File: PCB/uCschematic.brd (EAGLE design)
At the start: 90 x 80 mm, 63 parts, among them IC1 PIC24FJXXGA002/SO, IC10 ULN2003D1013TR, IC11 ULN2003D1013TR, IC12 ULN2003D1013TR, IC13 FT230XS-U, IC2 317EMP, IC3 MC74HC175ADG, IC4 MC74HC175ADG, IC5 MC74HC175ADG, IC6 MC74HC175ADG, IC7 MC74HC175ADG, IC8 MC74HC175ADG, IC9 ULN2003D1013TR, J1 UJ2-BH-1-TH, J8 68000-105HTLF, J9 68000-105HTLF, U1 74HC237D-Q100J

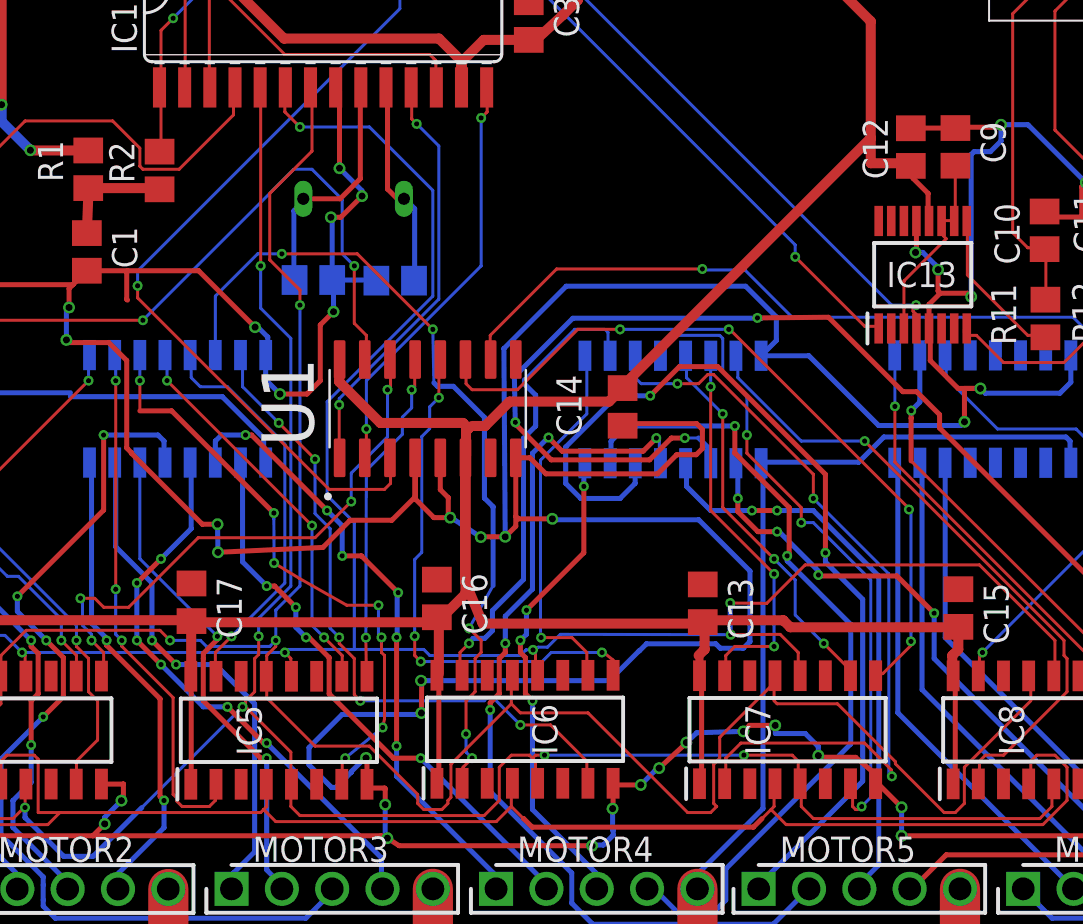
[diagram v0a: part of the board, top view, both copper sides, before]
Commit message: Ispravke u rutiranju
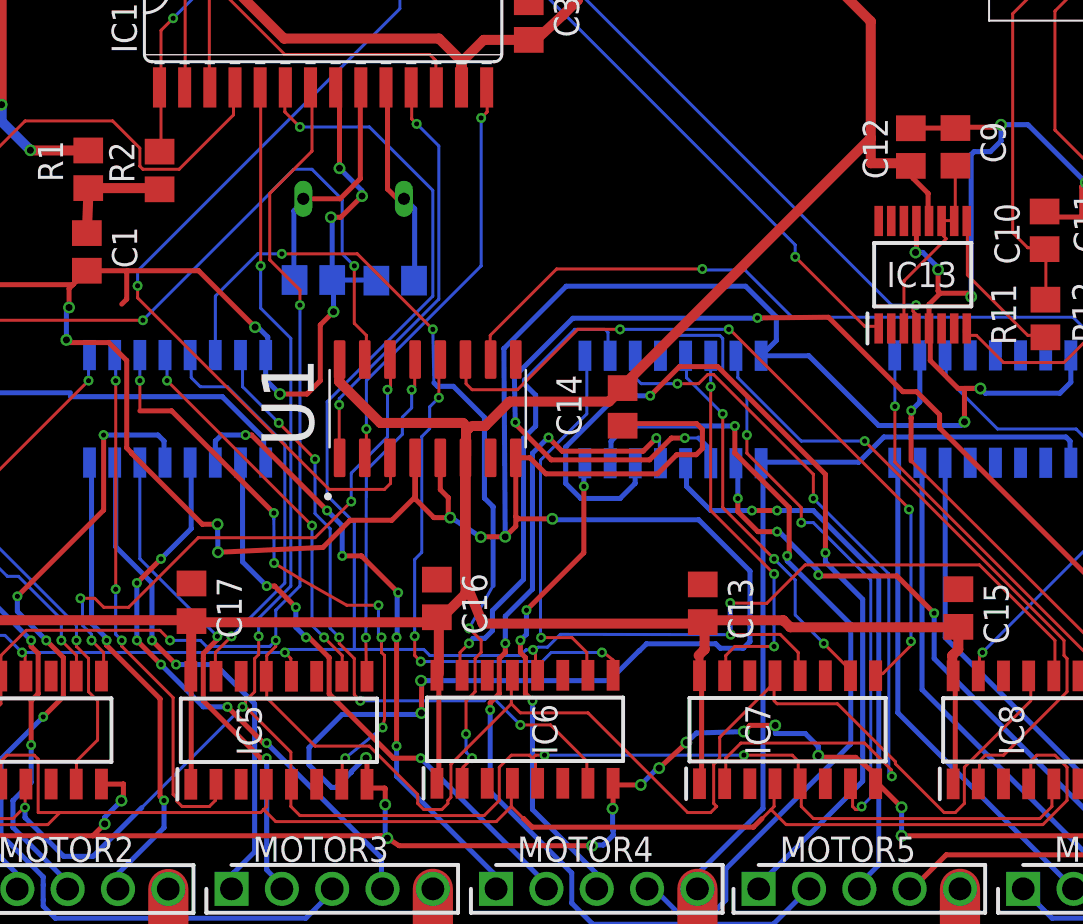
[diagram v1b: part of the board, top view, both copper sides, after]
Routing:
- net GND: track 500.6 -> 501.1 mm
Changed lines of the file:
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@@
 <?xml version="1.0" encoding="utf-8"?>
 <!DOCTYPE eagle SYSTEM "eagle.dtd">
-<eagle version="6.6.0">
+<eagle version="9.6.2">
 <drawing>
 <settings>
 <setting alwaysvectorfont="no"/>
+<setting keepoldvectorfont="yes"/>
 <setting verticaltext="up"/>
 </settings>
@@
 <param name="dpMaxLengthDifference" value="10mm"/>
 <param name="dpGapFactor" value="2.5"/>
-<param name="checkGrid" value="0"/>
 <param name="checkAngle" value="0"/>
 <param name="checkFont" value="1"/>
 <param name="checkRestrict" value="1"/>
+<param name="checkStop" value="0"/>
+<param name="checkValues" value="0"/>
+<param name="checkNames" value="1"/>
+<param name="checkWireStubs" value="1"/>
+<param name="checkPolygonWidth" value="0"/>
 <param name="useDiameter" value="13"/>
 <param name="maxErrors" value="50"/>
@@
 <pass name="Default">
 <param name="RoutingGrid" value="0.25mm"/>
+<param name="AutoGrid" value="1"/>
+<param name="Efforts" value="0"/>
+<param name="TopRouterVariant" value="1"/>
 <param name="tpViaShape" value="round"/>
 <param name="PrefDir.1" value="|"/>
@@
 <via x="20.20364375" y="9.065396875" extent="1-16" drill="0.35"/>
 <via x="27.5551375" y="9.661984375" extent="1-16" drill="0.35"/>
-<wire x1="28.39883125" y1="10.77141875" x2="28.39883125" y2="10.83833125" width="0.254" layer="16"/>
+<wire x1="28.39883125" y1="10.760046875" x2="28.39883125" y2="10.83833125" width="0.254" layer="16"/>
 <via x="28.39883125" y="10.83833125" extent="1-16" drill="0.35"/>
 <wire x1="28.39883125" y1="10.83833125" x2="28.49918125" y2="10.93868125" width="0.254" layer="1"/>
@@
 <wire x1="61.398775" y1="14.224465625" x2="61.3913375" y2="14.63620625" width="0.254" layer="16"/>
 <via x="61.3913375" y="14.63620625" extent="1-16" drill="0.35"/>
-<wire x1="59.676584375" y1="14.301878125" x2="59.7856" y2="14.33315" width="0.254" layer="1"/>
-<via x="59.7856" y="14.33315" extent="1-16" drill="0.35"/>
-<wire x1="59.7856" y1="14.33315" x2="57.432025" y2="14.263171875" width="0.254" layer="16"/>
-<wire x1="57.432025" y1="14.263171875" x2="56.906190625" y2="13.768446875" width="0.254" layer="16"/>
+<wire x1="59.693640625" y1="14.29050625" x2="59.80265625" y2="14.321778125" width="0.254" layer="1"/>
+<via x="59.80265625" y="14.321778125" extent="1-16" drill="0.35"/>
+<wire x1="59.80265625" y1="14.321778125" x2="57.4189875" y2="14.25090625" width="0.254" layer="16"/>
+<wire x1="57.4189875" y1="14.25090625" x2="56.906190625" y2="13.768446875" width="0.254" layer="16"/>
 <via x="56.906190625" y="13.768446875" extent="1-16" drill="0.35"/>
 <wire x1="56.906190625" y1="13.768446875" x2="56.75484375" y2="13.60516875" width="0.254" layer="1"/>
@@
 <wire x1="7.42666875" y1="57.50661875" x2="7.075165625" y2="57.858121875" width="0.254" layer="16"/>
 <wire x1="14.985165625" y1="47.508121875" x2="14.985165625" y2="49.41515" width="0.254" layer="16"/>
-<wire x1="61.3913375" y1="14.63620625" x2="60.08865625" y2="14.63620625" width="0.254" layer="1"/>
-<wire x1="60.08865625" y1="14.63620625" x2="59.7856" y2="14.33315" width="0.254" layer="1"/>
+<wire x1="61.3913375" y1="14.63620625" x2="60.117084375" y2="14.63620625" width="0.254" layer="1"/>
+<wire x1="60.117084375" y1="14.63620625" x2="59.80265625" y2="14.321778125" width="0.254" layer="1"/>
 <wire x1="15.005165625" y1="44.008121875" x2="15.005165625" y2="41.4866625" width="0.254" layer="16"/>
 <wire x1="15.005165625" y1="41.4866625" x2="15.055459375" y2="41.43636875" width="0.254" layer="16"/>
@@
 <wire x1="78.385225" y1="42.92861875" x2="78.385225" y2="46.080515625" width="0.254" layer="1"/>
 <wire x1="78.385225" y1="46.080515625" x2="82.582053125" y2="50.27734375" width="0.254" layer="1"/>
-<wire x1="70.67861875" y1="44.9429625" x2="70.47033125" y2="44.734675" width="0.254" layer="1"/>
-<wire x1="70.47033125" y1="44.734675" x2="70.47033125" y2="44.526284375" width="0.254" layer="1"/>
+<wire x1="70.78095" y1="45.113528125" x2="70.47033125" y2="44.802909375" width="0.254" layer="1"/>
+<wire x1="70.47033125" y1="44.802909375" x2="70.47033125" y2="44.526284375" width="0.254" layer="1"/>
 <wire x1="70.47033125" y1="44.526284375" x2="70.60911875" y2="44.526284375" width="0.254" layer="1"/>
 <wire x1="70.60911875" y1="44.526284375" x2="70.748046875" y2="44.6652125" width="0.254" layer="1"/>
@@
 <wire x1="28.900578125" y1="28.36699375" x2="28.900578125" y2="28.40045625" width="0.254" layer="1"/>
 <wire x1="28.900578125" y1="28.40045625" x2="28.666428125" y2="28.63460625" width="0.254" layer="1"/>
-<wire x1="28.70574375" y1="36.09621875" x2="28.66559375" y2="36.13636875" width="0.254" layer="1"/>
-<wire x1="28.66559375" y1="36.13636875" x2="28.66559375" y2="37.537971875" width="0.254" layer="1"/>
+<wire x1="28.415803125" y1="35.89154375" x2="28.66559375" y2="36.141334375" width="0.254" layer="1"/>
+<wire x1="28.66559375" y1="36.141334375" x2="28.66559375" y2="37.537971875" width="0.254" layer="1"/>
 <wire x1="28.66559375" y1="37.537971875" x2="28.70574375" y2="37.578121875" width="0.254" layer="1"/>
 <wire x1="28.666428125" y1="28.63460625" x2="28.666428125" y2="33.050275" width="0.254" layer="1"/>
@@
 <wire x1="57.828765625" y1="19.838921875" x2="57.828765625" y2="19.938921875" width="0.508" layer="1"/>
 <wire x1="57.523965625" y1="18.162521875" x2="57.828765625" y2="18.467321875" width="0.508" layer="1"/>
-<wire x1="57.523965625" y1="17.248121875" x2="57.570165625" y2="17.143121875" width="0.1524" layer="1"/>
+<wire x1="57.541090625" y1="17.172196875" x2="57.506909375" y2="17.15715625" width="0.1524" layer="1"/>
+<wire x1="57.541090625" y1="17.172196875" x2="57.570165625" y2="17.143121875" width="0.1524" layer="1"/>
 <wire x1="57.676365625" y1="17.095721875" x2="57.676365625" y2="11.761721875" width="0.254" layer="1"/>
 <wire x1="57.676365625" y1="11.761721875" x2="57.570165625" y2="11.693121875" width="0.1524" layer="1"/>
@@
 <wire x1="78.097965625" y1="18.162521875" x2="68.24776875" y2="27.9792875" width="0.1524" layer="1"/>
 <wire x1="78.097965625" y1="17.248121875" x2="78.097965625" y2="18.162521875" width="0.1524" layer="1"/>
-<wire x1="68.801565625" y1="33.250121875" x2="68.690165625" y2="33.310121875" width="0.1524" layer="16"/>
+<wire x1="68.79588125" y1="33.250121875" x2="68.6968" y2="33.3034875" width="0.1524" layer="16"/>
+<wire x1="68.6968" y1="33.3034875" x2="68.690165625" y2="33.310121875" width="0.1524" layer="16"/>
 <wire x1="78.097965625" y1="17.248121875" x2="77.990165625" y2="17.133121875" width="0.1524" layer="1"/>
 <via x="68.254" y="30.5171875" extent="1-16" drill="0.254"/>
@@
 </signal>
 </signals>
+<mfgpreviewcolors>
+<mfgpreviewcolor name="soldermaskcolor" color="0xC8008000"/>
+<mfgpreviewcolor name="silkscreencolor" color="0xFFFEFEFE"/>
+<mfgpreviewcolor name="backgroundcolor" color="0xFF282828"/>
+<mfgpreviewcolor name="coppercolor" color="0xFFFFBF00"/>
+<mfgpreviewcolor name="substratecolor" color="0xFF786E46"/>
+</mfgpreviewcolors>
 </board>
 </drawing>
